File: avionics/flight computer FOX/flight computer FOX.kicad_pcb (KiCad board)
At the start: 2 copper layers, 48.3 x 68.6 mm, 21 parts, among them J1 Screw_Terminal_01x02, J2 Conn_01x03, J3 Conn_01x03, J4 Conn_01x03, J5 Conn_01x03, J6 Conn_01x03, U1 ESP32-DevKitC, U2 LM7805_TO220

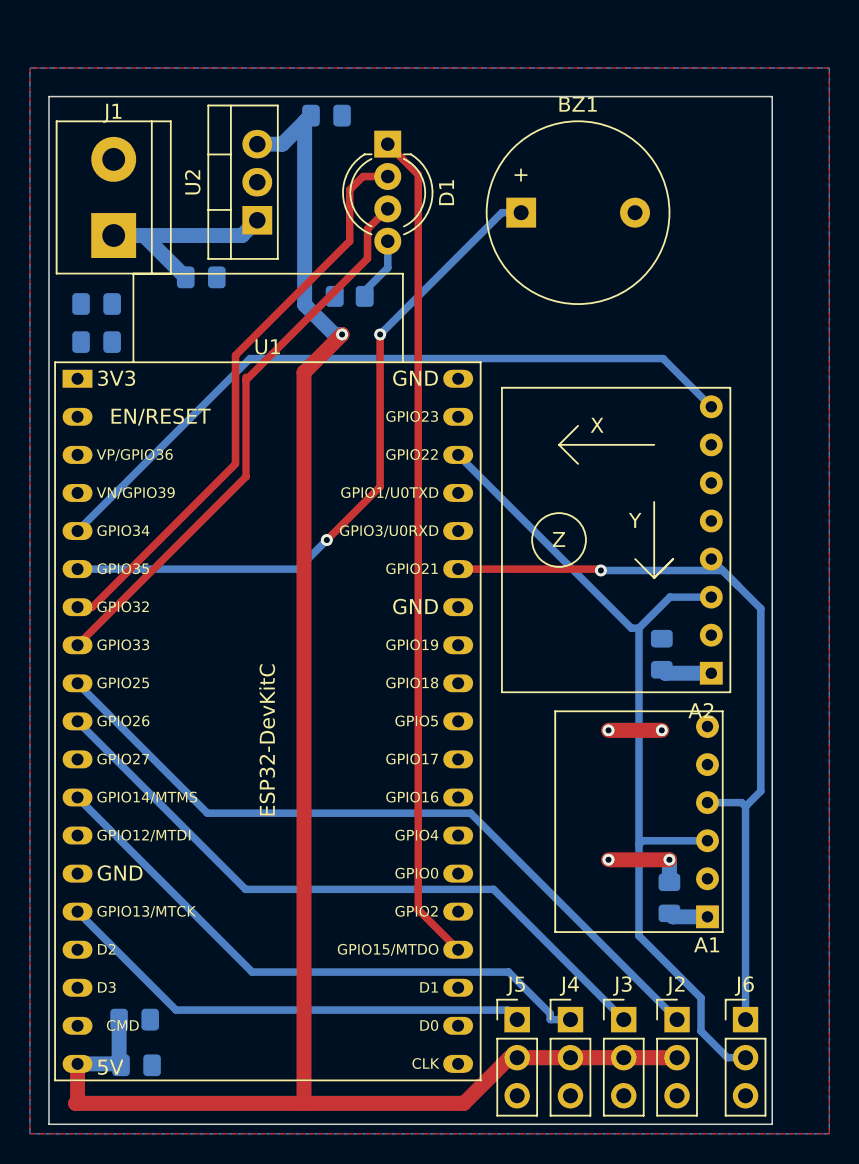
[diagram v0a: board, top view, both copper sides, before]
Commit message: lots of stuff
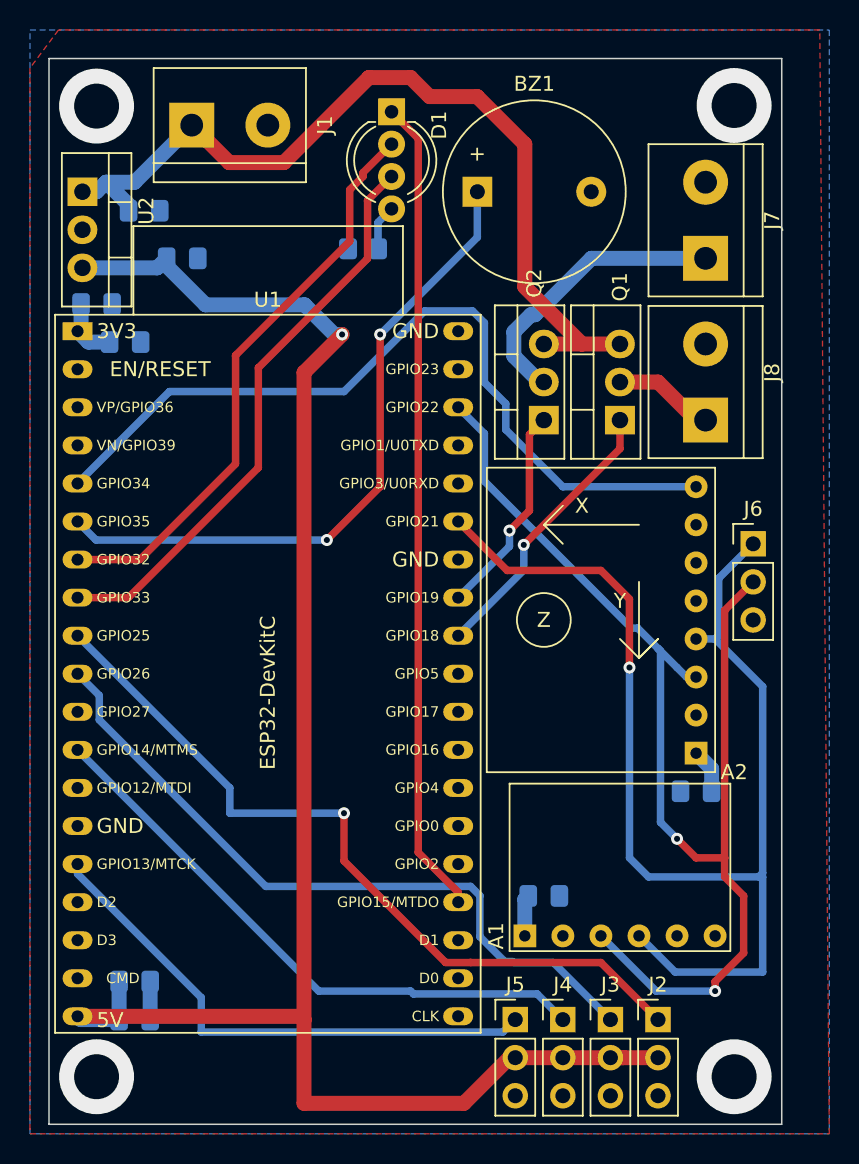
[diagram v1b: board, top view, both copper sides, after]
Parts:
- added J7: Screw_Terminal_01x02, TerminalBlock:TerminalBlock_bornier-2_P5.08mm, F.Cu at (70.5, 30.5)
- added J8: Screw_Terminal_01x02, TerminalBlock:TerminalBlock_bornier-2_P5.08mm, F.Cu at (70.5, 41.3)
- added Q1: IRF540N, Package_TO_SOT_THT:TO-220-3_Vertical, F.Cu at (64.8, 41.3)
- added Q2: IRF540N, Package_TO_SOT_THT:TO-220-3_Vertical, F.Cu at (59.7, 41.3)
- moved J6 31.8 mm to (73.7, 49.5)
- moved C8 13.5 mm to (35.6, 30.5)
- moved A1 12.3 mm to (58.4, 75.7), turned to 90 degrees
- moved U2 11.8 mm to (28.9, 26.0), turned to -90 degrees
- moved C6 9.43 mm to (69.8, 66.0), turned to 180 degrees
- moved J1 9.02 mm to (36.2, 21.6), turned to 0 degrees
- moved C5 8.38 mm to (59.7, 73.0), turned to 0 degrees
- moved C7 5.85 mm to (33.0, 27.3)
- moved C2 5.59 mm to (32.4, 78.7)
- moved A2 5.43 mm to (69.8, 63.5)
- moved R1 3.30 mm to (47.6, 29.8)
- moved BZ1 3.24 mm to (55.3, 26.0)
- moved U1 3.17 mm to (28.6, 35.3)
- moved D1 2.17 mm to (49.5, 20.7)
- moved C1 1.91 mm to (31.8, 36.1)
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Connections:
- U1 pad 30: unconnected-(U1-GPIO18-Pad30) -> pyro1
- U1 pad 31: unconnected-(U1-GPIO19-Pad31) -> pyro2
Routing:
- net +BATT: track 16.0 -> 59.1 mm
- net SDA: track 54.3 -> 81.8 mm
- net SCL: track 59.5 -> 80.7 mm, vias 0 -> 2
- net pyro2out: track 0.00 -> 19.2 mm
- net pyro1: track 0.00 -> 18.9 mm, vias 0 -> 1
- net pyro2: track 0.00 -> 14.2 mm, vias 0 -> 1
- net pyro1out: track 0.00 -> 6.77 mm
- net INTMPU: track 48.4 -> 54.2 mm
- net +5V: track 123.0 -> 118.7 mm
- net +3V3: track 6.03 -> 10.1 mm
- net servoout4: track 32.3 -> 35.9 mm
- net GND: track 9.12 -> 5.66 mm
- net servoout2: track 44.7 -> 47.7 mm
- net servoout1: track 49.3 -> 52.2 mm, vias 0 -> 1
- net Net-(D1-K): track 4.32 -> 3.04 mm
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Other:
- board size 48.3 x 68.6 mm -> 48.9 x 71.1 mm
